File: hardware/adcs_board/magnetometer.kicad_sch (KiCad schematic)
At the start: 66 parts, among them T3 IRF7105TR, T4 IRF7105TR, U25 HMC1002-TR, U26 LM324NSR, U27 HMC1001-RC, U28 ADS1257IRGWT, U5 MT3608, U6 MT3608, U7 LM324NSR

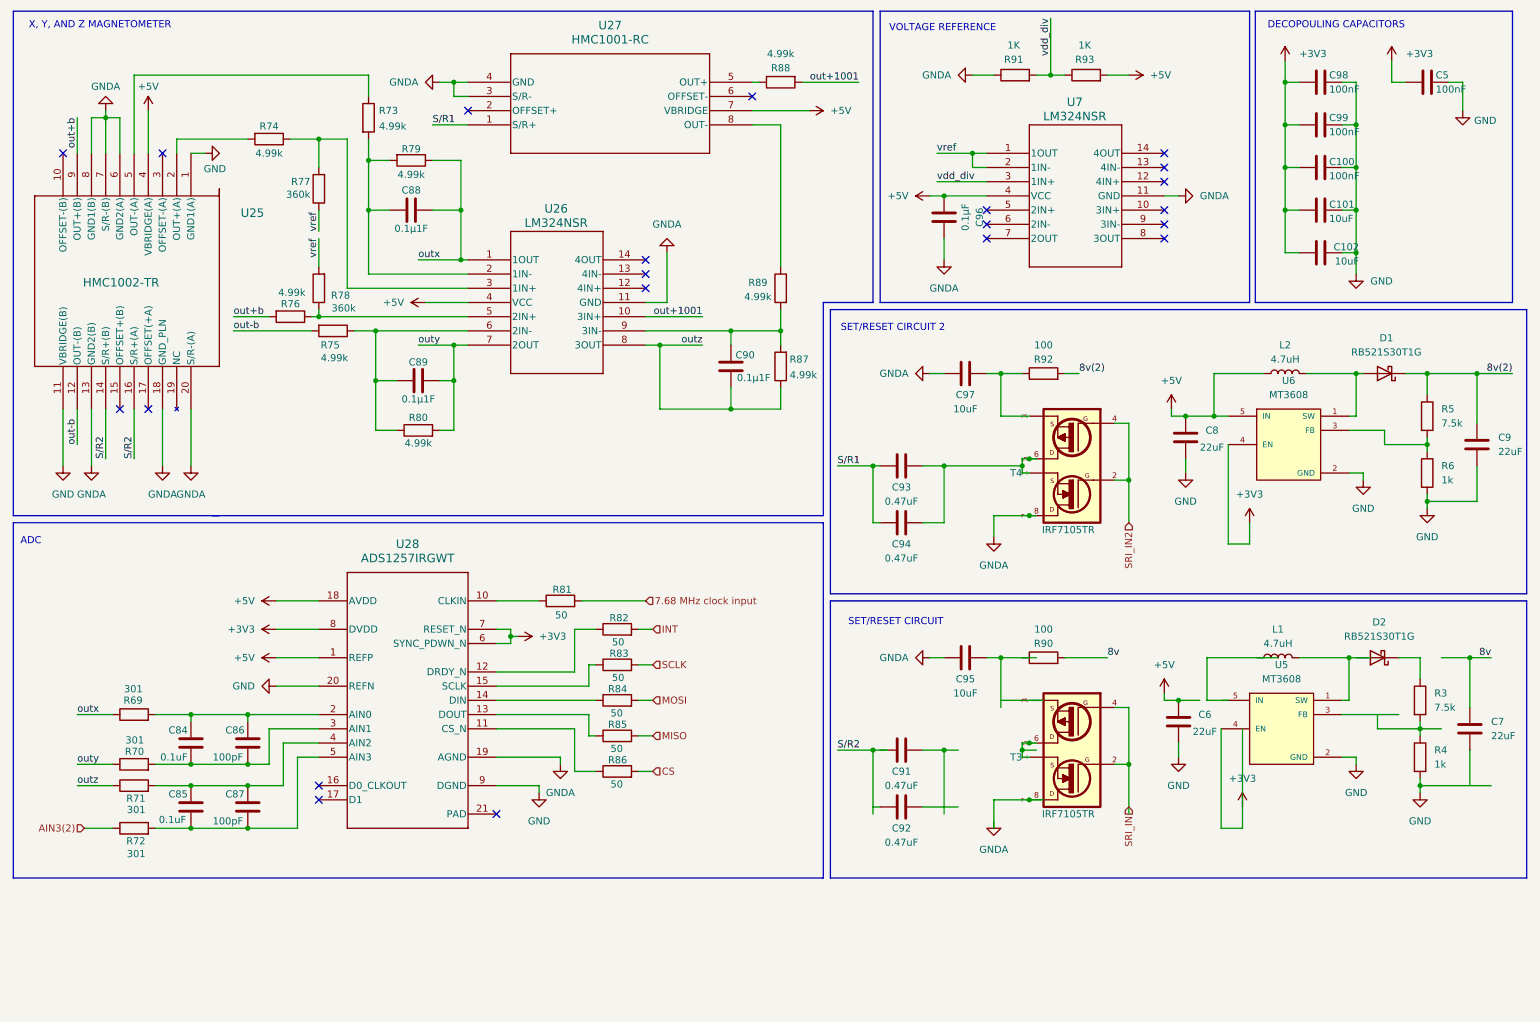
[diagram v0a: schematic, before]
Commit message: hardware: schematic and layout fixes
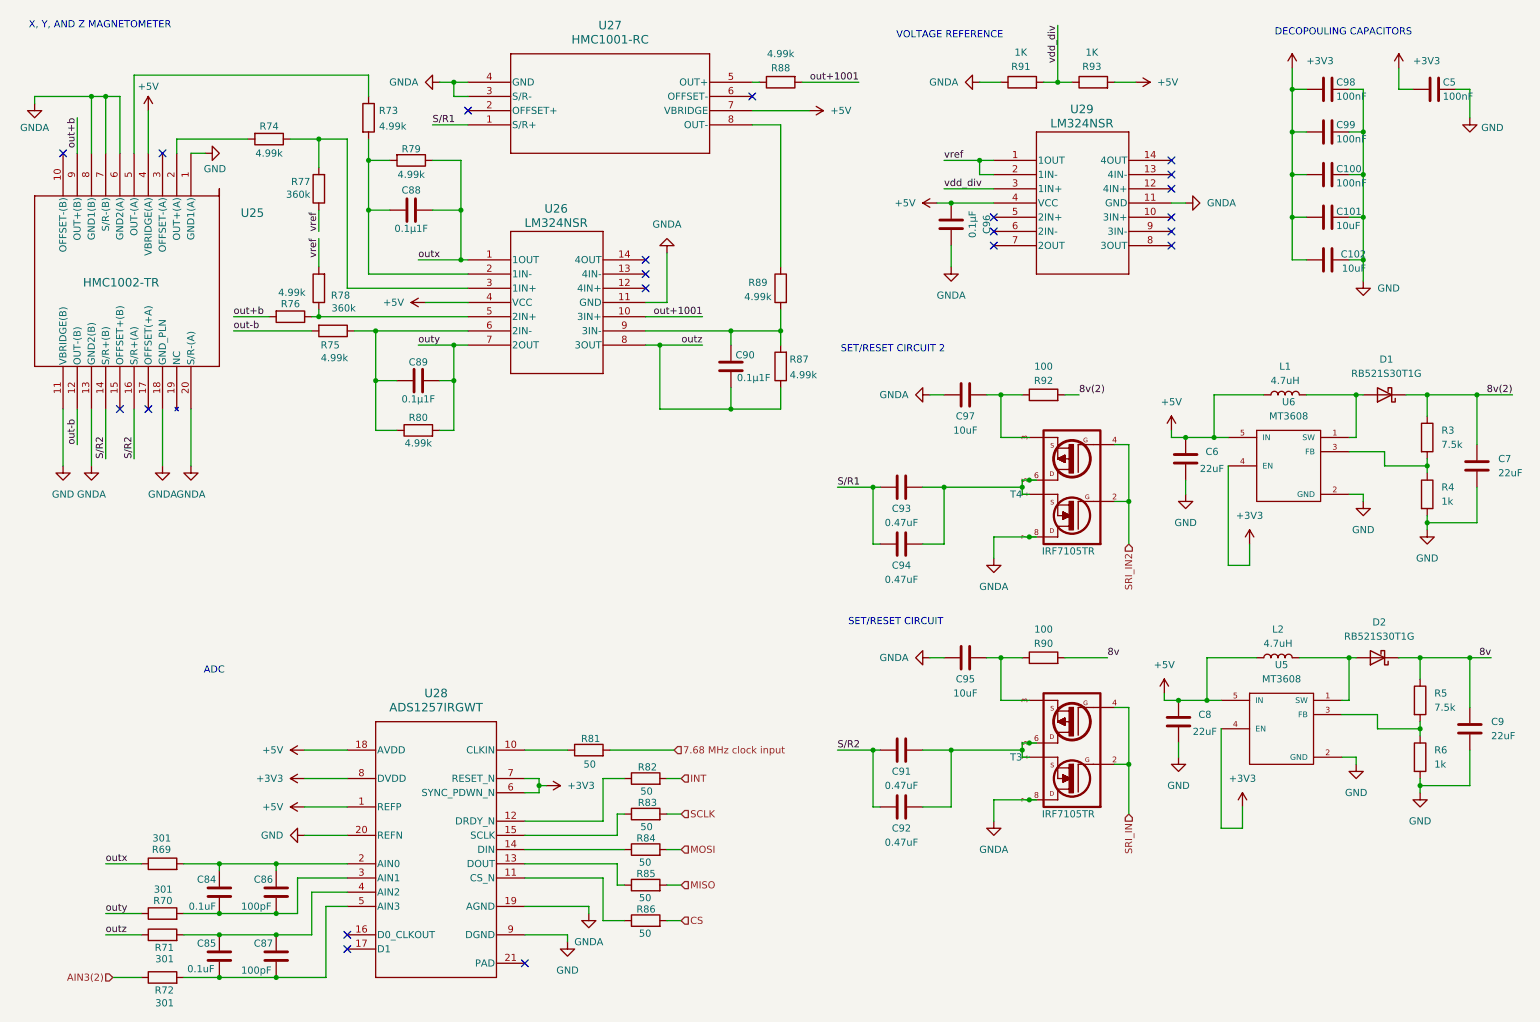
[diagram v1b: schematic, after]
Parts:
- renumbered C8 to C6, C9 to C7, C6 to C8, C7 to C9, L2 to L1, L1 to L2, R5 to R3, R6 to R4, R3 to R5, R4 to R6, U7 to U29
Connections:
- net +3V3: now also U5.4 (EN)
- net +5V: now also L2.1, U5.5 (IN)
- net 8v: now also D2.1 (K), R5.1
- net GND: now also C9.2
- net GNDA: now also T3.7, T3.8
- net S/R2: now also C91.1, C92.1
- net at C92.2: now also C91.2, T3.1, T3.5, T3.6
- net at L2.2, U5.1 (SW): now also D2.2 (A)
- net at R5.2, R6.1: now also U5.3 (FB)
- net at T3.3: now also C95.2, R90.1
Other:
- moved on the sheet: C100, C101, C102, C5, C6, C7, C84, C85, C86, C87, C93, C94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
